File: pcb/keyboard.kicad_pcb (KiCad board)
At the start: 2 copper layers, 331.1 x 102 mm, 139 parts, among them J1 USB_C_Receptacle_USB2.0, Q1 BC858, SW1 SW_Push, SW10 SW_Push, SW11 SW_Push, SW12 SW_Push, SW13 SW_Push, SW14 SW_Push, SW15 SW_Push, SW16 SW_Push, SW17 SW_Push, SW18 SW_Push, SW19 SW_Push, SW2 SW_Push, SW20 SW_Push, SW21 SW_Push, SW22 SW_Push, SW23 SW_Push, SW24 SW_Push, SW25 SW_Push, SW26 SW_Push, SW27 SW_Push, SW28 SW_Push, SW29 SW_Push, SW3 SW_Push, SW30 SW_Push, SW31 SW_Push, SW32 SW_Push, SW33 SW_Push, SW34 SW_Push, SW35 SW_Push, SW36 SW_Push, SW37 SW_Push, SW38 SW_Push, SW39 SW_Push, SW4 SW_Push, SW40 SW_Push, SW41 SW_Push, SW42 SW_Push, SW43 SW_Push, SW44 SW_Push, SW45 SW_Push, SW46 SW_Push, SW47 SW_Push, SW48 SW_Push, SW49 SW_Push, SW5 SW_Push, SW50 SW_Push, SW6 SW_Push, SW7 SW_Push, SW8 SW_Push, SW9 SW_Push, U1 NCP1117-3.3_SOT223, U2 USBLC6-2SC6, U3 W25Q128JVS, U4 RP2040, Y1 ABM8-272_T3

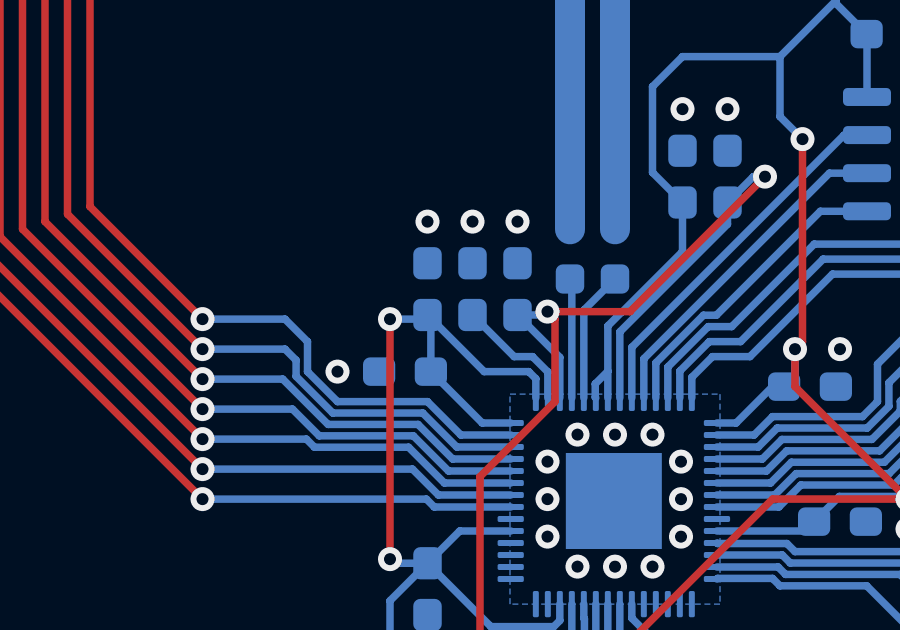
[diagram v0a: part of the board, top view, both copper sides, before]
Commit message: Ready to produce test production files before updating some components
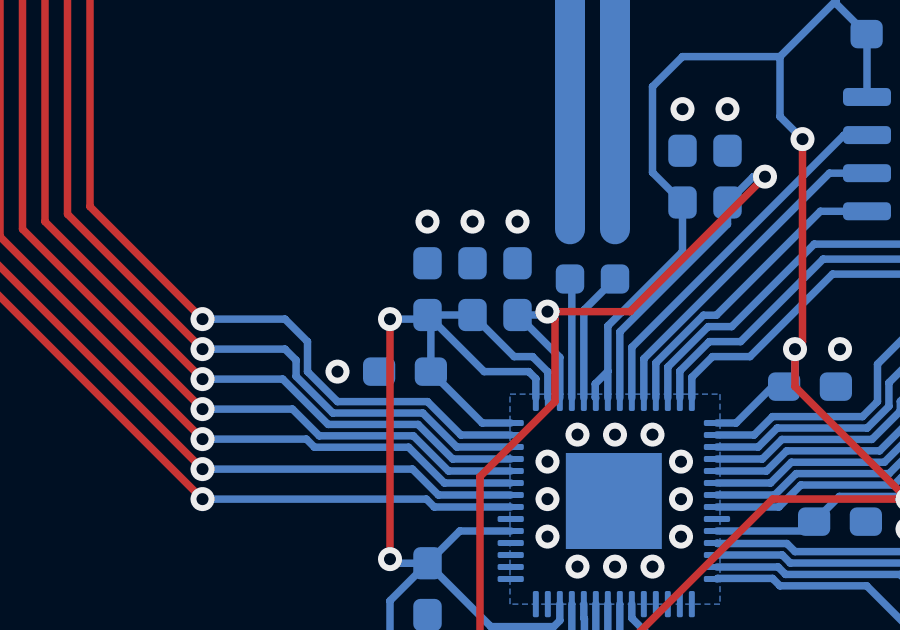
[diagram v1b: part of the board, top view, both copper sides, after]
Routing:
- net +3V3: track 147.4 -> 148.9 mm
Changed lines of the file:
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@@
   (segment (start 217.75 145) (end 216.5375 146.2125) (width 0.25) (layer "B.Cu") (net 3))
   (segment (start 209.1375 144) (end 207.75 142.6125) (width 0.25) (layer "B.Cu") (net 3))
+  (segment (start 206.25 142.6125) (end 207.75 142.6125) (width 0.25) (layer "B.Cu") (net 3))
   (segment (start 219.8625 132.1375) (end 218 134) (width 0.25) (layer "B.Cu") (net 3))
   (segment (start 208.075 146.2125) (end 206.3625 144.5) (width 0.25) (layer "B.Cu") (net 3))
